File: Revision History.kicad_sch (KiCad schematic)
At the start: 0 parts

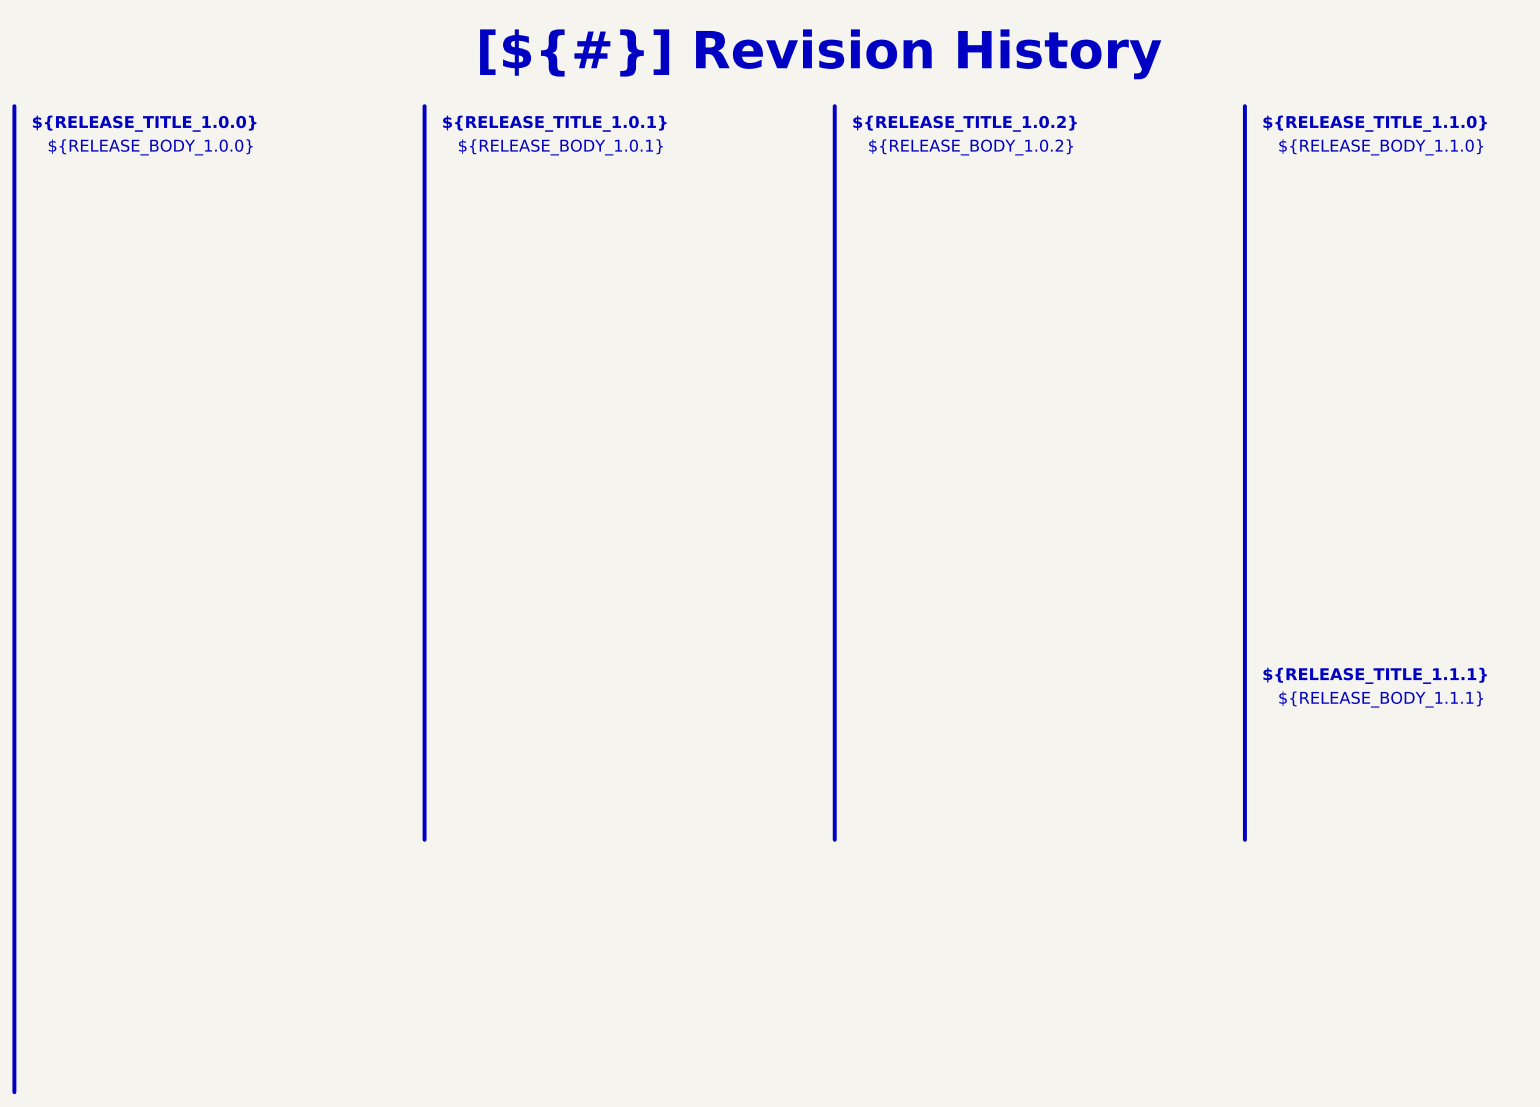
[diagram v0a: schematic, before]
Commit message: Kicad 10
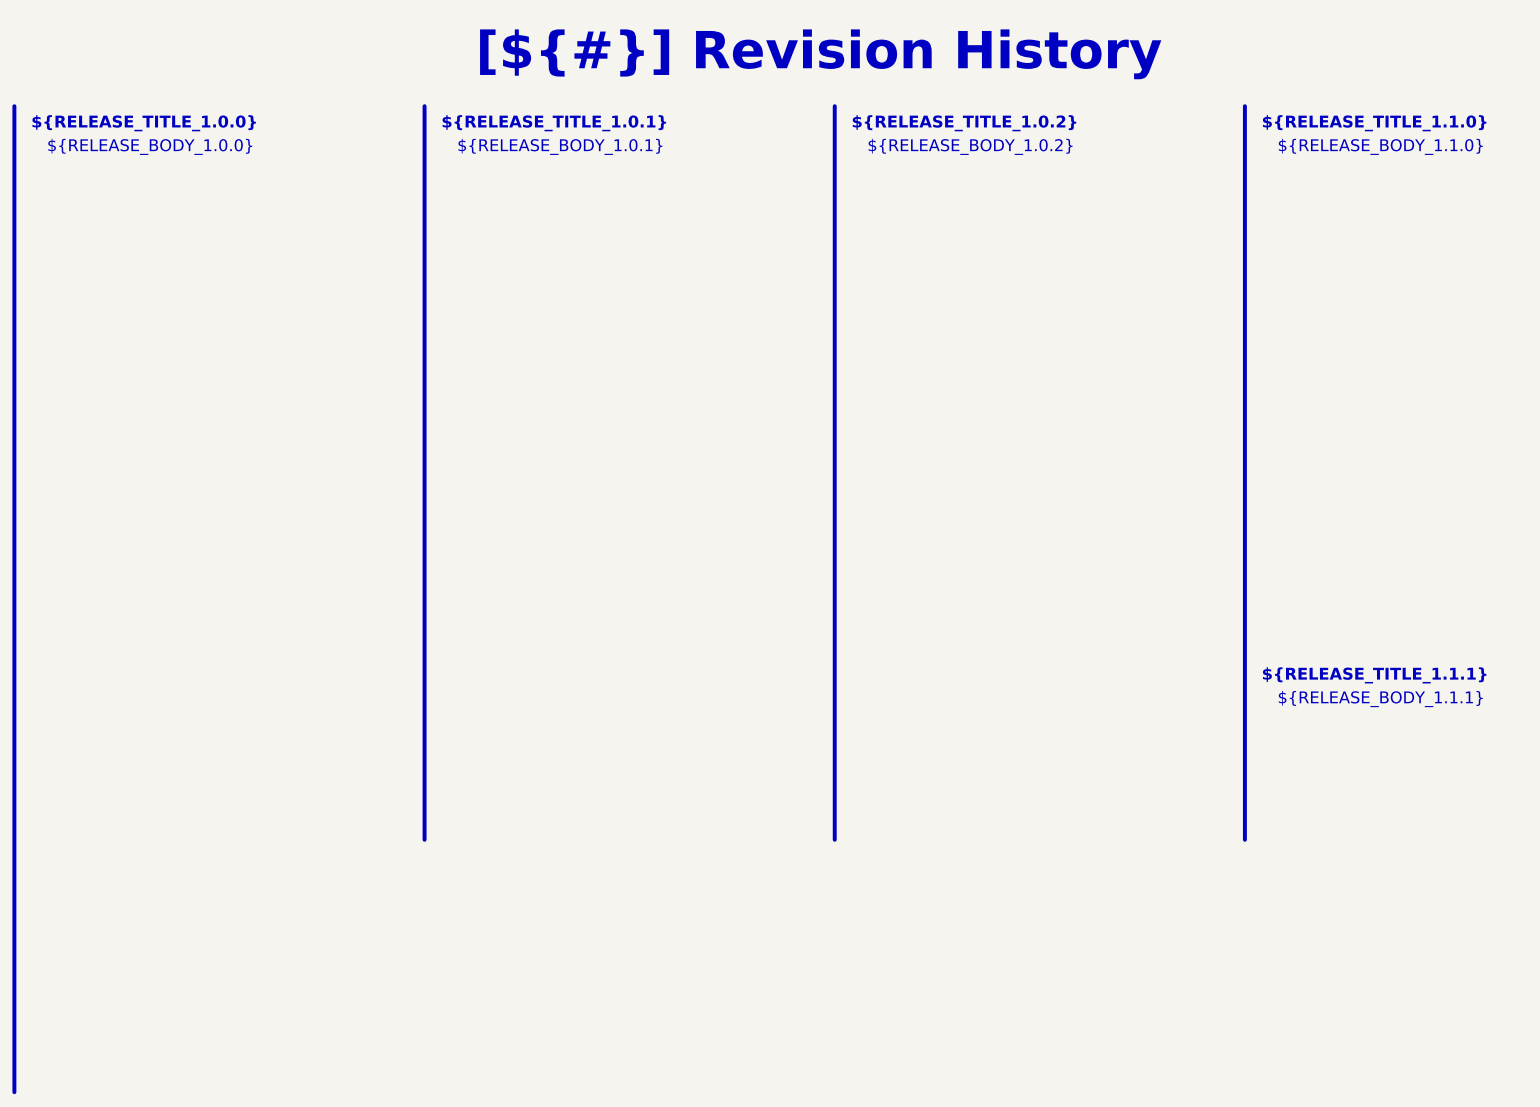
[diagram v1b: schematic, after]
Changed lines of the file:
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@@
 (kicad_sch
-	(version 20231120)
+	(version 20260306)
 	(generator "eeschema")
-	(generator_version "8.0")
+	(generator_version "10.0")
 	(paper "A4")
 	(title_block
@@
 		(company "${COMPANY}")
 	)
-	(polyline
-		(pts
-			(xy 85.09 31.75) (xy 85.09 149.86)
-		)
-		(stroke
-			(width 0.635)
-			(type default)
-			(color 0 0 0 1)
-		)
-	)
-	(polyline
-		(pts
-			(xy 151.13 31.75) (xy 151.13 149.86)
-		)
-		(stroke
-			(width 0.635)
-			(type default)
-			(color 0 0 0 1)
-		)
-	)
-	(polyline
-		(pts
-			(xy 19.05 31.75) (xy 19.05 190.5)
-		)
-		(stroke
-			(width 0.635)
-			(type default)
-			(color 0 0 0 1)
-		)
-	)
-	(polyline
-		(pts
-			(xy 217.17 31.75) (xy 217.17 149.86)
-		)
-		(stroke
-			(width 0.635)
-			(type default)
-			(color 0 0 0 1)
-		)
-	)
 	(text_box "${RELEASE_BODY_1.1.0}"
 		(exclude_from_sim no)
 		(at 220.98 35.56 0)
 		(size 58.42 81.28)
+		(margins 1.4287 1.4287 1.4287 1.4287)
 		(stroke
 			(width -0.0001)
@@
 		(at 80.01 16.51 0)
 		(size 137.16 12.7)
+		(margins 4.4999 4.4999 4.4999 4.4999)
 		(stroke
 			(width -0.0001)
@@
 		(at 22.86 35.56 0)
 		(size 58.42 146.05)
+		(margins 1.4287 1.4287 1.4287 1.4287)
 		(stroke
 			(width -0.0001)
@@
 		(at 152.4 31.75 0)
 		(size 57.15 7.62)
+		(margins 1.4287 1.4287 1.4287 1.4287)
 		(stroke
 			(width -0.0001)
@@
 		(at 220.98 124.46 0)
 		(size 58.42 24.13)
+		(margins 1.4287 1.4287 1.4287 1.4287)
 		(stroke
 			(width -0.0001)
@@
 		(at 218.44 120.65 0)
 		(size 57.15 7.62)
+		(margins 1.4287 1.4287 1.4287 1.4287)
 		(stroke
 			(width -0.0001)
@@
 		(at 154.94 35.56 0)
 		(size 58.42 111.76)
+		(margins 1.4287 1.4287 1.4287 1.4287)
 		(stroke
 			(width -0.0001)
@@
 		(at 88.9 35.56 0)
 		(size 57.15 105.41)
+		(margins 1.4287 1.4287 1.4287 1.4287)
 		(stroke
 			(width -0.0001)
@@
 		(at 20.32 31.75 0)
 		(size 57.15 7.62)
+		(margins 1.4287 1.4287 1.4287 1.4287)
 		(stroke
 			(width -0.0001)
@@
 		(at 86.36 31.75 0)
 		(size 57.15 7.62)
+		(margins 1.4287 1.4287 1.4287 1.4287)
 		(stroke
 			(width -0.0001)
@@
 		(at 218.44 31.75 0)
 		(size 57.15 7.62)
-		(stroke
-			(width -0.0001)
-			(type default)
-		)
-		(fill
-			(type none)
-		)
-		(effects
-			(font
-				(face "Arial")
-				(size 1.905 1.905)
-				(thickness 0.254)
-				(bold yes)
-			)
-			(justify left top)
-		)
-	)
+		(margins 1.4287 1.4287 1.4287 1.4287)
+		(stroke
+			(width -0.0001)
+			(type default)
+		)
+		(fill
+			(type none)
+		)
+		(effects
+			(font
+				(face "Arial")
+				(size 1.905 1.905)
+				(thickness 0.254)
+				(bold yes)
+			)
+			(justify left top)
+		)
+	)
+	(polyline
+		(pts
+			(xy 85.09 31.75) (xy 85.09 149.86)
+		)
+		(stroke
+			(width 0.635)
+			(type default)
+			(color 0 0 0 1)
+		)
+	)
+	(polyline
+		(pts
+			(xy 151.13 31.75) (xy 151.13 149.86)
+		)
+		(stroke
+			(width 0.635)
+			(type default)
+			(color 0 0 0 1)
+		)
+	)
+	(polyline
+		(pts
+			(xy 19.05 31.75) (xy 19.05 190.5)
+		)
+		(stroke
+			(width 0.635)
+			(type default)
+			(color 0 0 0 1)
+		)
+	)
+	(polyline
+		(pts
+			(xy 217.17 31.75) (xy 217.17 149.86)
+		)
+		(stroke
+			(width 0.635)
+			(type default)
+			(color 0 0 0 1)
+		)
+	)
